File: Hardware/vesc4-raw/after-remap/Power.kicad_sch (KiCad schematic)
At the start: 48 parts, among them U2 TC2117, U3 DRV8302

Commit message: export footprint & ngapus warning unmatched
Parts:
- C1: symbol after-remap-rescue:C-RESCUE-BLDC_4 -> vesc4-legacy:C-RESCUE-BLDC_4_28
- C18: symbol after-remap-rescue:C-RESCUE-BLDC_4 -> vesc4-legacy:C-RESCUE-BLDC_4_48
- C19: symbol after-remap-rescue:C-RESCUE-BLDC_4 -> vesc4-legacy:C-RESCUE-BLDC_4_44
- C20: symbol after-remap-rescue:C-RESCUE-BLDC_4 -> vesc4-legacy:C-RESCUE-BLDC_4_46
- C21: symbol after-remap-rescue:C-RESCUE-BLDC_4 -> vesc4-legacy:C-RESCUE-BLDC_4_45
- C22: symbol after-remap-rescue:C-RESCUE-BLDC_4 -> vesc4-legacy:C-RESCUE-BLDC_4_50
- C23: symbol after-remap-rescue:C-RESCUE-BLDC_4 -> vesc4-legacy:C-RESCUE-BLDC_4_43
- C24: symbol after-remap-rescue:C-RESCUE-BLDC_4 -> vesc4-legacy:C-RESCUE-BLDC_4_26
- C25: symbol after-remap-rescue:CP1-RESCUE-BLDC_4 -> vesc4-legacy:CP1-RESCUE-BLDC_4_4
- C26: symbol after-remap-rescue:C-RESCUE-BLDC_4 -> vesc4-legacy:C-RESCUE-BLDC_4_49
- C27: symbol after-remap-rescue:C-RESCUE-BLDC_4 -> vesc4-legacy:C-RESCUE-BLDC_4_37
- C28: symbol after-remap-rescue:C-RESCUE-BLDC_4 -> vesc4-legacy:C-RESCUE-BLDC_4_35
- C29: symbol after-remap-rescue:C-RESCUE-BLDC_4 -> vesc4-legacy:C-RESCUE-BLDC_4_38
- C30: symbol after-remap-rescue:C-RESCUE-BLDC_4 -> vesc4-legacy:C-RESCUE-BLDC_4_33
- C33: symbol after-remap-rescue:CP1-RESCUE-BLDC_4 -> vesc4-legacy:CP1-RESCUE-BLDC_4_3
- C34: symbol after-remap-rescue:C-RESCUE-BLDC_4 -> vesc4-legacy:C-RESCUE-BLDC_4_36
- C36: symbol after-remap-rescue:C-RESCUE-BLDC_4 -> vesc4-legacy:C-RESCUE-BLDC_4_34
- C37: symbol after-remap-rescue:C-RESCUE-BLDC_4 -> vesc4-legacy:C-RESCUE-BLDC_4_29
- C39: symbol after-remap-rescue:C-RESCUE-BLDC_4 -> vesc4-legacy:C-RESCUE-BLDC_4_39
- C40: symbol after-remap-rescue:C-RESCUE-BLDC_4 -> vesc4-legacy:C-RESCUE-BLDC_4_30
- C43: symbol after-remap-rescue:C-RESCUE-BLDC_4 -> vesc4-legacy:C-RESCUE-BLDC_4_40
- C44: symbol after-remap-rescue:C-RESCUE-BLDC_4 -> vesc4-legacy:C-RESCUE-BLDC_4_41
- C49: symbol after-remap-rescue:C-RESCUE-BLDC_4 -> vesc4-legacy:C-RESCUE-BLDC_4_42
- C51: symbol after-remap-rescue:C-RESCUE-BLDC_4 -> vesc4-legacy:C-RESCUE-BLDC_4_32
- C52: symbol after-remap-rescue:C-RESCUE-BLDC_4 -> vesc4-legacy:C-RESCUE-BLDC_4_47
- C8: symbol after-remap-rescue:C-RESCUE-BLDC_4 -> vesc4-legacy:C-RESCUE-BLDC_4_27
- C9: symbol after-remap-rescue:C-RESCUE-BLDC_4 -> vesc4-legacy:C-RESCUE-BLDC_4_31
- D4: symbol after-remap-rescue:DIODESCH -> vesc4-legacy:DIODESCH_2
- D5: symbol after-remap-rescue:DIODE -> vesc4-legacy:DIODE_2
- L1: symbol after-remap-rescue:INDUCTOR -> vesc4-legacy:INDUCTOR_2
- R17: symbol after-remap-rescue:R-RESCUE-BLDC_4 -> vesc4-legacy:R-RESCUE-BLDC_4_29
- R18: symbol after-remap-rescue:R-RESCUE-BLDC_4 -> vesc4-legacy:R-RESCUE-BLDC_4_31
- R19: symbol after-remap-rescue:R-RESCUE-BLDC_4 -> vesc4-legacy:R-RESCUE-BLDC_4_28
- R20: symbol after-remap-rescue:R-RESCUE-BLDC_4 -> vesc4-legacy:R-RESCUE-BLDC_4_32
- R21: symbol after-remap-rescue:R-RESCUE-BLDC_4 -> vesc4-legacy:R-RESCUE-BLDC_4_30
- R23: symbol after-remap-rescue:R-RESCUE-BLDC_4 -> vesc4-legacy:R-RESCUE-BLDC_4_23
- R24: symbol after-remap-rescue:R-RESCUE-BLDC_4 -> vesc4-legacy:R-RESCUE-BLDC_4_22
- R25: symbol after-remap-rescue:R-RESCUE-BLDC_4 -> vesc4-legacy:R-RESCUE-BLDC_4_21
- R26: symbol after-remap-rescue:R-RESCUE-BLDC_4 -> vesc4-legacy:R-RESCUE-BLDC_4_26
- R27: symbol after-remap-rescue:R-RESCUE-BLDC_4 -> vesc4-legacy:R-RESCUE-BLDC_4_27
- R32: symbol after-remap-rescue:R-RESCUE-BLDC_4 -> vesc4-legacy:R-RESCUE-BLDC_4_24
- R33: symbol after-remap-rescue:R-RESCUE-BLDC_4 -> vesc4-legacy:R-RESCUE-BLDC_4_25
- R48: symbol after-remap-rescue:R-RESCUE-BLDC_4 -> vesc4-legacy:R-RESCUE-BLDC_4_17
- R49: symbol after-remap-rescue:R-RESCUE-BLDC_4 -> vesc4-legacy:R-RESCUE-BLDC_4_18
- R50: symbol after-remap-rescue:R-RESCUE-BLDC_4 -> vesc4-legacy:R-RESCUE-BLDC_4_19
- R51: symbol after-remap-rescue:R-RESCUE-BLDC_4 -> vesc4-legacy:R-RESCUE-BLDC_4_20
- U2: symbol after-remap-rescue:NCP1117ST33T3G -> vesc4-legacy:NCP1117ST33T3G_2
- U3: symbol after-remap-rescue:DRV8302 -> vesc4-legacy:DRV8302_2

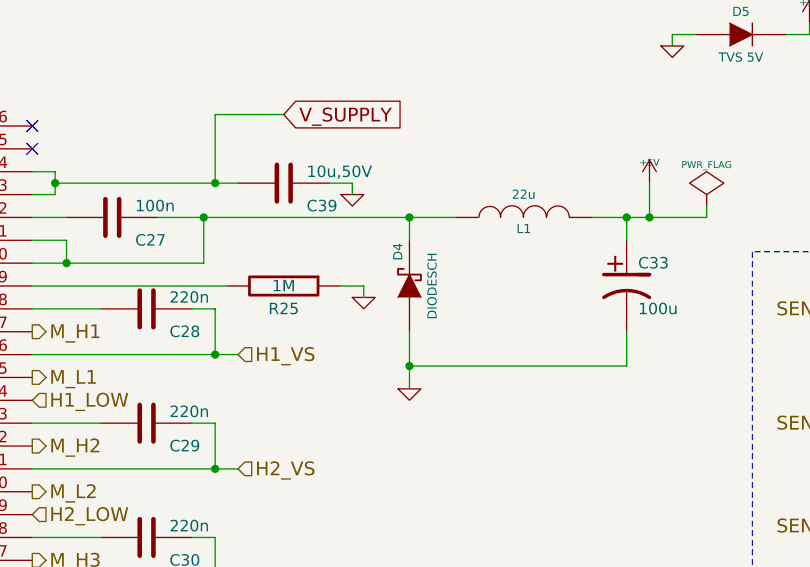
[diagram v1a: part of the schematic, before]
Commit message: checkpoint sebelum ngetrace usb
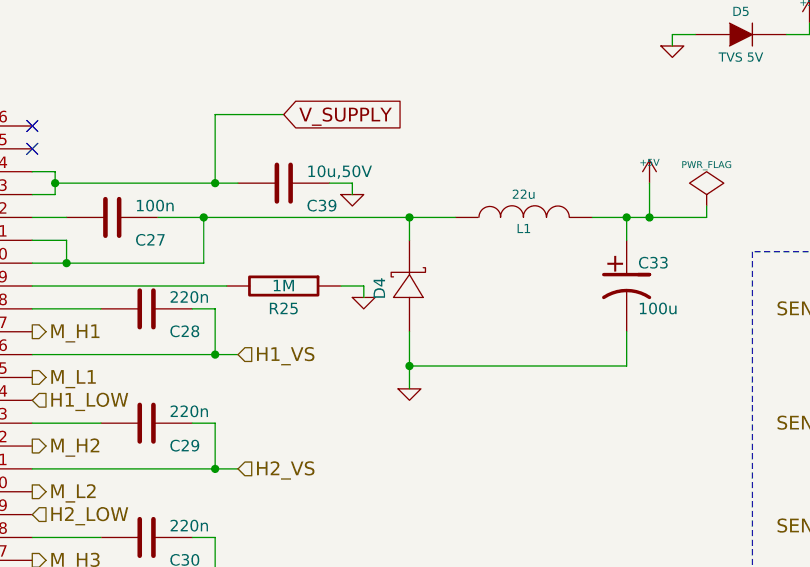
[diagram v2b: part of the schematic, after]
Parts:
- removed D4: DIODESCH, Diodes_SMD:SMA_Handsoldering, symbol vesc4-legacy:DIODESCH_2
- added D4: ~, EasyEDA_Lib:SMA_L4.2-W2.6-LS5.1-RD, symbol EasyEDA_Lib:SS110_C379823
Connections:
- net GND: now also D4.2 (A)
- net at C27.1, L1.1, U3.50 (PH)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: now also D4.1 (K)
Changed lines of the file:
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@@
 	)
 	(symbol
-		(lib_name "DIODESCH_2")
-		(lib_id "vesc4-legacy:DIODESCH_2")
-		(at 198.12 82.55 90)
-		(unit 1)
-		(exclude_from_sim no)
-		(in_bom yes)
-		(on_board yes)
-		(dnp no)
-		(property "Reference" "D4"
-			(at 196.85 78.74 0)
-			(effects
-				(font
-					(size 1.016 1.016)
-				)
-			)
-		)
-		(property "Value" "DIODESCH"
-			(at 200.66 82.55 0)
-			(effects
-				(font
-					(size 1.016 1.016)
-				)
-			)
-		)
-		(property "Footprint" "Diodes_SMD:SMA_Handsoldering"
-			(at 198.12 82.55 0)
-			(effects
-				(font
-					(size 1.524 1.524)
-				)
-				(hide yes)
-			)
-		)
-		(property "Datasheet" ""
-			(at 198.12 82.55 0)
-			(effects
-				(font
-					(size 1.524 1.524)
-				)
-				(hide yes)
-			)
-		)
-		(property "Description" ""
-			(at 198.12 82.55 0)
-			(effects
-				(font
-					(size 1.27 1.27)
-				)
-			)
-		)
-		(pin "1"
-		)
-		(pin "2"
-		)
-		(instances
-			(project "after-remap"
-				(path "/97cdaedc-7981-4798-95b0-56b9c66aae09/00000000-0000-0000-0000-0000504f83be"
-					(reference "D4")
-					(unit 1)
-				)
-			)
-		)
-	)
-	(symbol
 		(lib_name "R-RESCUE-BLDC_4_23")
 		(lib_id "vesc4-legacy:R-RESCUE-BLDC_4_23")
@@
 					(unit 1)
 				)
+			)
+		)
+	)
+	(symbol
+		(lib_id "EasyEDA_Lib:SS110_C379823")
+		(at 198.12 82.55 270)
+		(unit 1)
+		(exclude_from_sim no)
+		(in_bom yes)
+		(on_board yes)
+		(dnp no)
+		(property "Reference" "D4"
+			(at 194.818 82.804 0)
+			(effects
+				(font
+					(size 1.27 1.27)
+				)
+			)
+		)
+		(property "Value" "~"
+			(at 194.31 82.169 0)
+			(effects
+				(font
+					(size 1.27 1.27)
+				)
+			)
+		)
+		(property "Footprint" "EasyEDA_Lib:SMA_L4.2-W2.6-LS5.1-RD"
+			(at 198.12 82.55 0)
+			(effects
+				(font
+					(size 1.27 1.27)
+				)
+				(hide yes)
+			)
+		)
+		(property "Datasheet" "https://atta.szlcsc.com/upload/public/pdf/source/20190416/C379823_9D66F8781E151C8A4940396CFA0EFE63.pdf"
+			(at 198.12 82.55 0)
+			(effects
+				(font
+					(size 1.27 1.27)
+				)
+				(hide yes)
+			)
+		)
+		(property "Description" "Forward Voltage (Vf@If):850mV@1A Reverse Voltage (Vr):100V Average Rectified Current (Io):1A"
+			(at 198.12 82.55 0)
+			(effects
+				(font
+					(size 1.27 1.27)
+				)
+				(hide yes)
+			)
+		)
+		(property "Manufacturer Part" "SS110"
+			(at 198.12 82.55 0)
+			(effects
+				(font
+					(size 1.27 1.27)
+				)
+				(hide yes)
+			)
+		)
+		(property "Supplier Part" "C379823"
+			(at 198.12 82.55 0)
+			(effects
+				(font
+					(size 1.27 1.27)
+				)
+				(hide yes)
+			)
+		)
+		(property "Supplier" "LCSC"
+			(at 198.12 82.55 0)
+			(effects
+				(font
+					(size 1.27 1.27)
+				)
+				(hide yes)
+			)
+		)
+		(property "LCSC Part Name" "电压:100V 电流:1A"
+			(at 198.12 82.55 0)
+			(effects
+				(font
+					(size 1.27 1.27)
+				)
+				(hide yes)
+			)
+		)
+		(pin "1"
+		)
+		(pin "2"
+		)
+		(instances
+			(project "after-remap"
+				(path "/97cdaedc-7981-4798-95b0-56b9c66aae09/00000000-0000-0000-0000-0000504f83be"
+					(reference "D4")
+					(unit 1)
+				)

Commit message: changed inductor
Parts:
- L1: footprint w_smd_inductors:inductor_smd_8x5mm -> Library:IND-SMD_L6.0-W6.0-shield
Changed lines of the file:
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@@
 			)
 		)
-		(property "Footprint" "w_smd_inductors:inductor_smd_8x5mm"
+		(property "Footprint" "Library:IND-SMD_L6.0-W6.0-shield"
 			(at 210.82 74.93 0)
 			(effects

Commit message: changed c tantalum
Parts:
- C25, C33: footprint w_smd_cap:c_tant_B -> Library:CAP-SMD_L3.5-W2.8-R-RD
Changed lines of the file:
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@@
 			)
 		)
-		(property "Footprint" "w_smd_cap:c_tant_B"
+		(property "Footprint" "Library:CAP-SMD_L3.5-W2.8-R-RD"
 			(at 222.25 82.55 0)
 			(effects
@@
 			)
 		)
-		(property "Footprint" "w_smd_cap:c_tant_B"
+		(property "Footprint" "Library:CAP-SMD_L3.5-W2.8-R-RD"
 			(at 182.88 35.56 0)
 			(effects

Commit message: changed 15u 100V footprint
c37 c51
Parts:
- C37, C51: footprint w_smd_cap:c_2220 -> Library:C2220_L5.6-W5.0-H3.0
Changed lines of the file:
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@@
 			)
 		)
-		(property "Footprint" "w_smd_cap:c_2220"
+		(property "Footprint" "Library:C2220_L5.6-W5.0-H3.0"
 			(at 231.14 35.56 0)
 			(effects
@@
 			)
 		)
-		(property "Footprint" "w_smd_cap:c_2220"
+		(property "Footprint" "Library:C2220_L5.6-W5.0-H3.0"
 			(at 270.51 36.83 0)
 			(effects

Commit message: sebelum ganti kapasitor 1206
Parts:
- C40, C43, C44, C49, C9: footprint CRF1:SMD-1206 -> Library:C1206
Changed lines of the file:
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@@
 			)
 		)
-		(property "Footprint" "CRF1:SMD-1206"
+		(property "Footprint" "Library:C1206"
 			(at 149.86 152.4 0)
 			(effects
@@
 			)
 		)
-		(property "Footprint" "CRF1:SMD-1206"
+		(property "Footprint" "Library:C1206"
 			(at 149.86 158.75 0)
 			(effects
@@
 			)
 		)
-		(property "Footprint" "CRF1:SMD-1206"
+		(property "Footprint" "Library:C1206"
 			(at 149.86 165.1 0)
 			(effects
@@
 			)
 		)
-		(property "Footprint" "CRF1:SMD-1206"
+		(property "Footprint" "Library:C1206"
 			(at 231.14 30.48 0)
 			(effects
@@
 			)
 		)
-		(property "Footprint" "CRF1:SMD-1206"
+		(property "Footprint" "Library:C1206"
 			(at 231.14 25.4 0)
 			(effects

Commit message: changed footprint 4n7 cap
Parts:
- C23: footprint CRF1:SMD-0603_c -> Library:C0603
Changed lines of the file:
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@@
 			)
 		)
-		(property "Footprint" "CRF1:SMD-0603_c"
+		(property "Footprint" "Library:C0603"
 			(at 105.41 138.43 0)
 			(effects
